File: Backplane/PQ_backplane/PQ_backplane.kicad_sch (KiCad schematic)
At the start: 12 parts, among them J1 M55-6002642R, J2 M55-6003242R, J3 M55-6002642R, J4 M55-6001242R, J5 USB4110-GF-A, U4 FUSB302BMPX

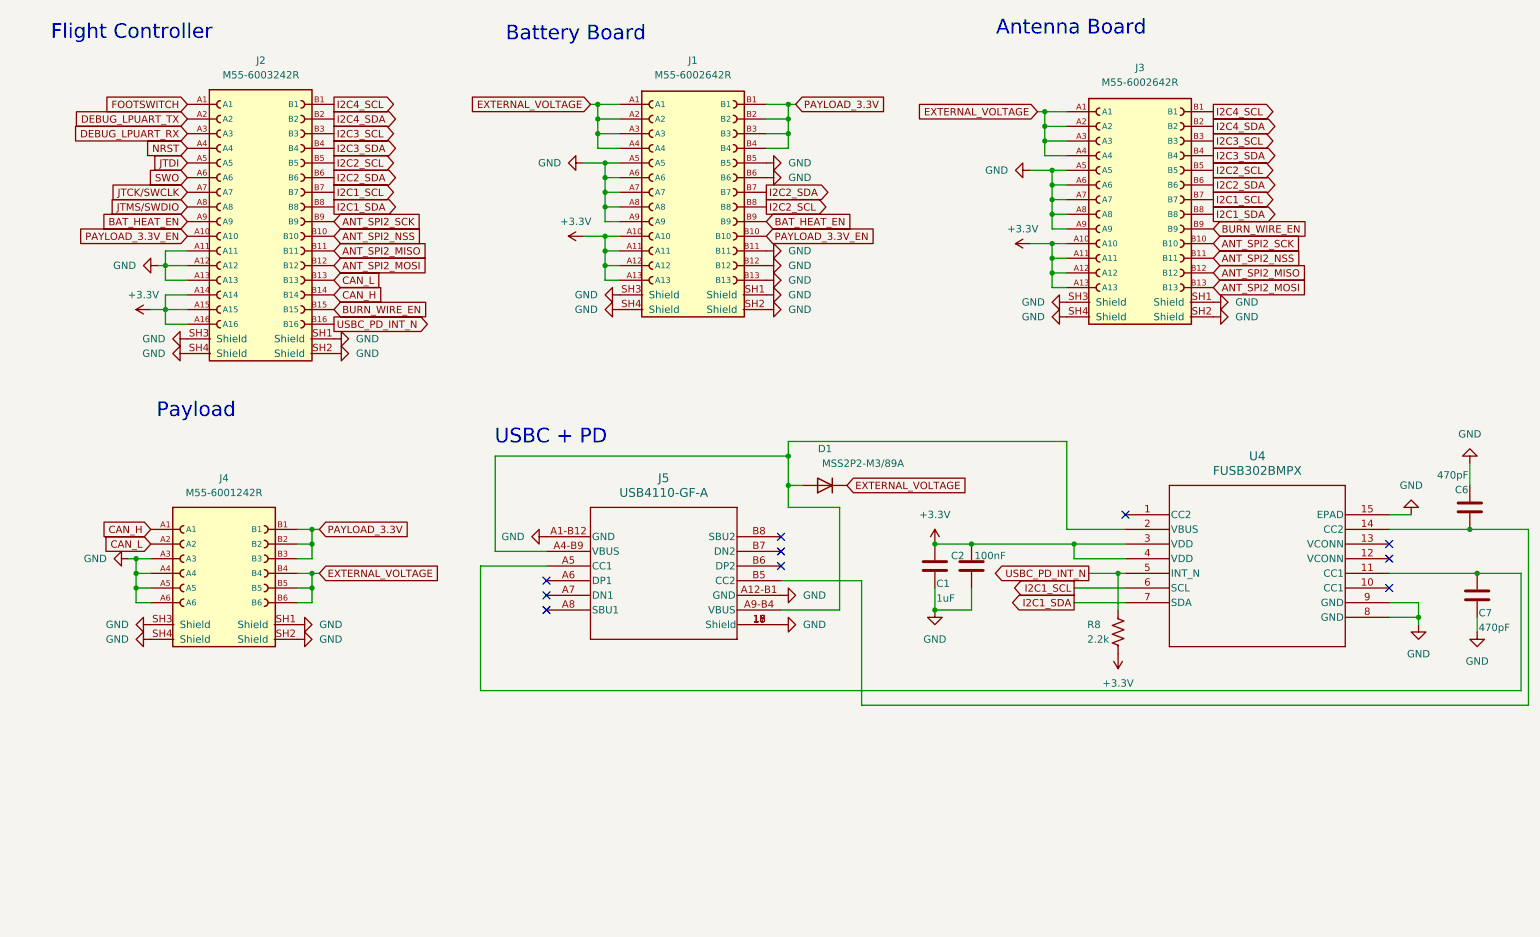
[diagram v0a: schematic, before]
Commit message: Pushing changes to backplane
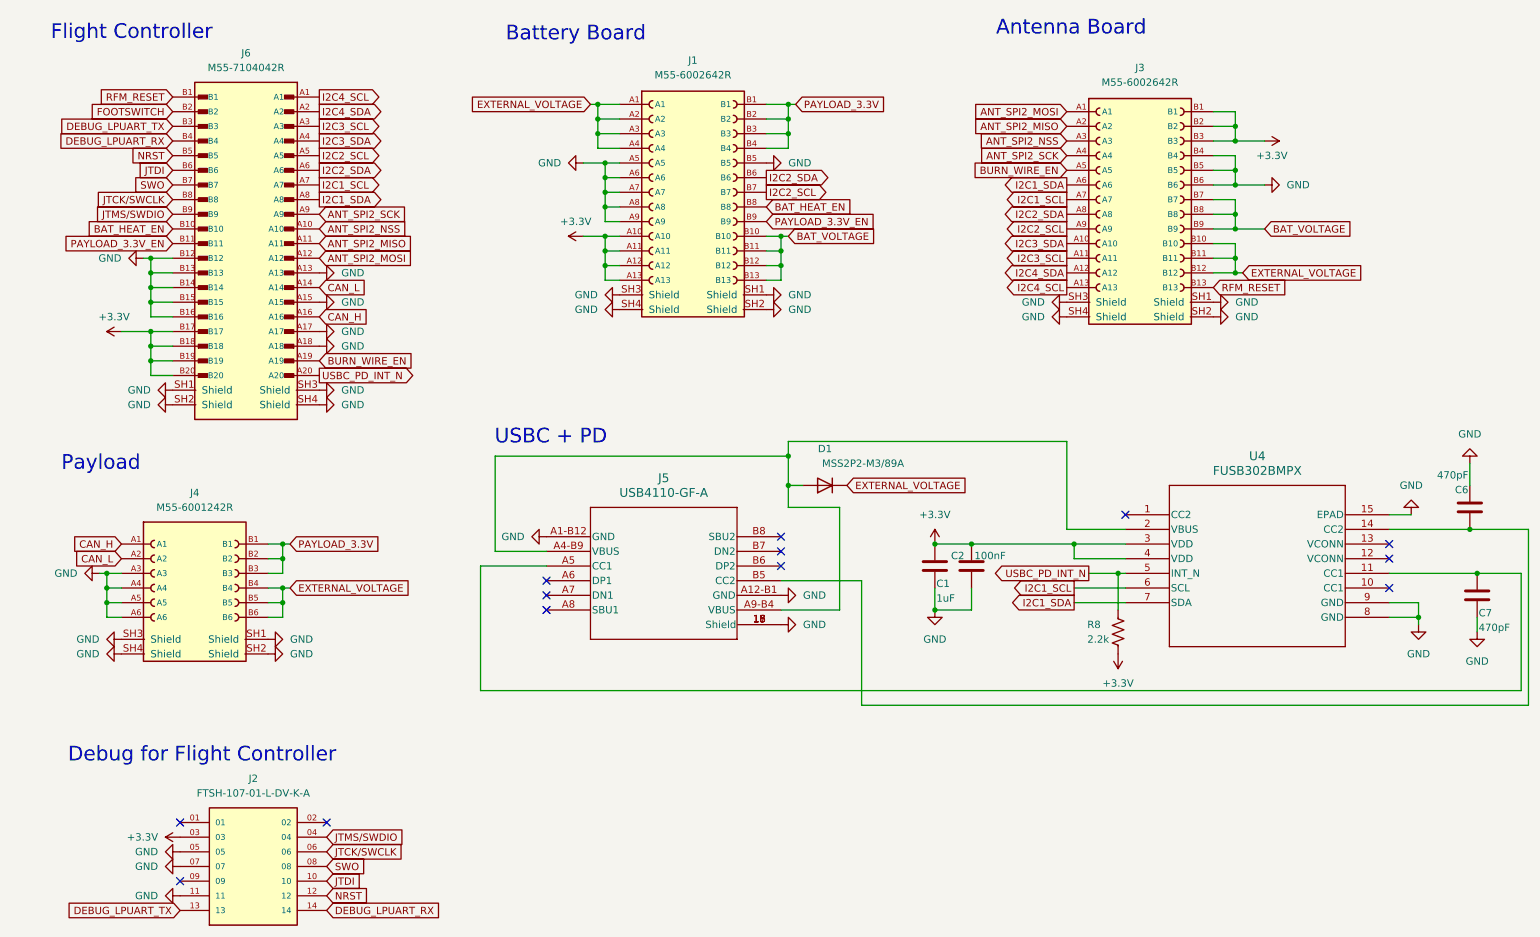
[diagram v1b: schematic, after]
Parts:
- removed J2: M55-6003242R, inspireflyFootPrints:HARWIN_M55-6003242R, symbol inspireflySym:M55-6003242R
- added J2: FTSH-107-01-L-DV-K-A, inspireflyFootPrints:SAMTEC_FTSH-107-01-L-DV-K-A, symbol inspirefly:FTSH-107-01-L-DV-K-A
- added J6: M55-7104042R, inspireflyFootPrints:HARWIN_M55-7104042R, symbol inspirefly:M55-7104042R
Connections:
- net +3.3V: now also J3.B1, J3.B2, J3.B3, J2.03, J6.B17, J6.B18, J6.B19, J6.B20; no longer J3.A10, J3.A11, J3.A12, J3.A13
- net ANT_SPI2_MISO: now also J3.A2, J6.A11; no longer J3.B12
- net ANT_SPI2_MOSI: now also J3.A1, J6.A12; no longer J3.B13
- net ANT_SPI2_NSS: now also J3.A3, J6.A10; no longer J3.B11
- net ANT_SPI2_SCK: now also J3.A4, J6.A9; no longer J3.B10
- net BAT_HEAT_EN: now also J1.B8, J6.B10; no longer J1.B9
- net BURN_WIRE_EN: now also J3.A5, J6.A19; no longer J3.B9
- net CAN_H: now also J6.A16
- net CAN_L: now also J6.A14
- net DEBUG_LPUART_RX: now also J2.14, J6.B4
- net DEBUG_LPUART_TX: now also J2.13, J6.B3
- net EXTERNAL_VOLTAGE: now also J3.B10, J3.B11, J3.B12; no longer J3.A1, J3.A2, J3.A3, J3.A4
- net FOOTSWITCH: now also J6.B2
- net GND: now also J3.B4, J3.B5, J3.B6, J2.05, J2.07, J2.11, J6.A13, J6.A15, J6.A17, J6.A18, J6.B12, J6.B13, J6.B14, J6.B15, J6.B16, J6.SH1 (Shield), J6.SH2 (Shield), J6.SH3 (Shield), J6.SH4 (Shield); no longer J1.B11, J1.B12, J1.B13, J1.B6, J3.A5, J3.A6, J3.A7, J3.A8, J3.A9
- net I2C1_SCL: now also J3.A7, J6.A7; no longer J3.B7
- net I2C1_SDA: now also J3.A6, J6.A8; no longer J3.B8
- net I2C2_SCL: now also J1.B7, J3.A9, J6.A5; no longer J1.B8, J3.B5
- net I2C2_SDA: now also J1.B6, J3.A8, J6.A6; no longer J1.B7, J3.B6
- net I2C3_SCL: now also J3.A11, J6.A3; no longer J3.B3
- net I2C3_SDA: now also J3.A10, J6.A4; no longer J3.B4
- net I2C4_SCL: now also J3.A13, J6.A1; no longer J3.B1
- net I2C4_SDA: now also J3.A12, J6.A2; no longer J3.B2
- net JTCK/SWCLK: now also J2.06, J6.B8
- net JTDI: now also J2.10, J6.B6
- net JTMS/SWDIO: now also J2.04, J6.B9
- net NRST: now also J2.12, J6.B5
- net PAYLOAD_3.3V_EN: now also J1.B9, J6.B11; no longer J1.B10
- net SWO: now also J2.08, J6.B7
- net USBC_PD_INT_N: now also J6.A20
- new net BAT_VOLTAGE: J1.B10, J1.B11, J1.B12, J1.B13, J3.B7, J3.B8, J3.B9
- new net RFM_RESET: J3.B13, J6.B1
- no-connect marks 10 -> 13
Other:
- note added: "Debug for Flight Controller"
- moved on the sheet: J4
